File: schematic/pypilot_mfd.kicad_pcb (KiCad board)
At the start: 2 copper layers, 115.8 x 85.9 mm, 72 parts, among them J1 usb, J2 keypad, J3 Conn_01x02, J4 Conn_01x02, J5 jlx256160, J6 usb, J7 uart, Q1 Q_PMOS_GSD, Q2 Q_PMOS_GSD, Q3 Q_PMOS_DSG, SW1 BOOT/AP, U1 CH340G, U2 AMS1117-3.3, U3 ESP32-WROOM-32D, U5 ADM2587E, U6 LIS2DE12, U7 74AHC04, U8 BUZZER-freetronics_schematic, Y1 12mhz

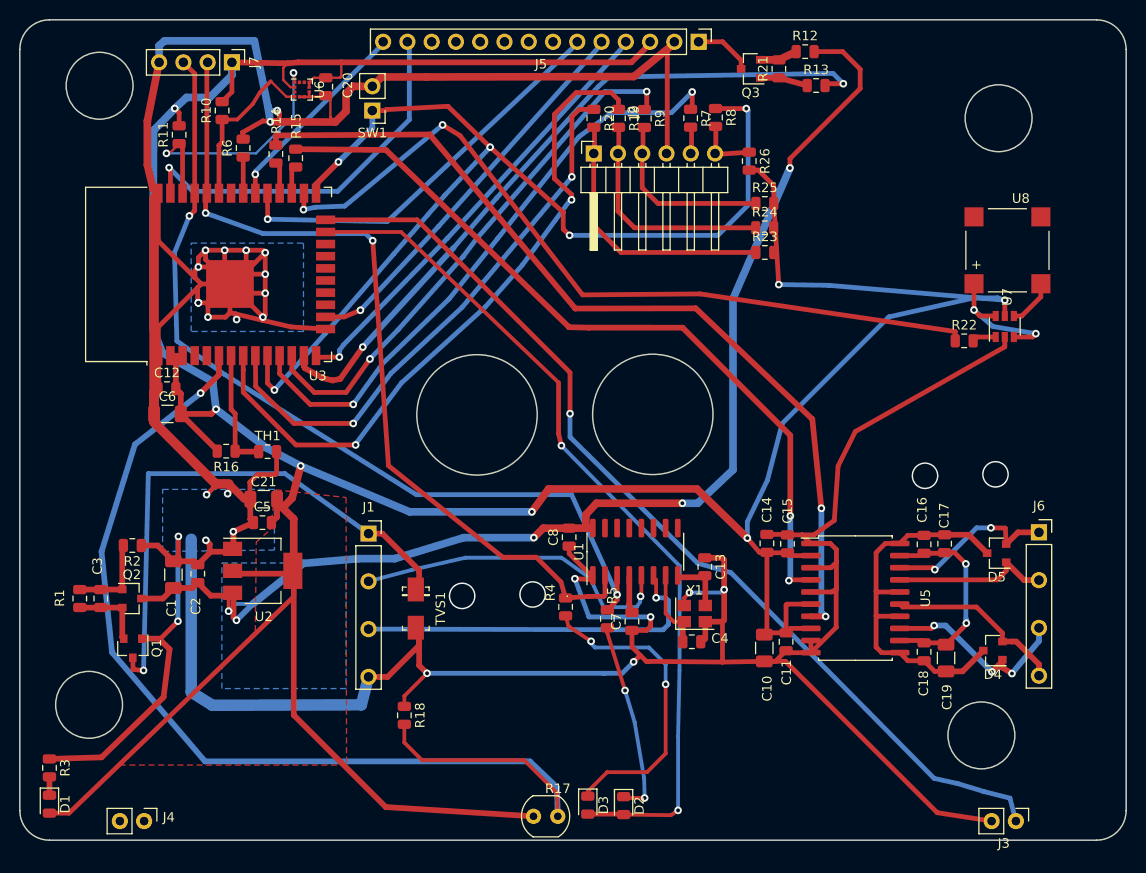
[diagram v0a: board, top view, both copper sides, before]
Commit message: many updates!
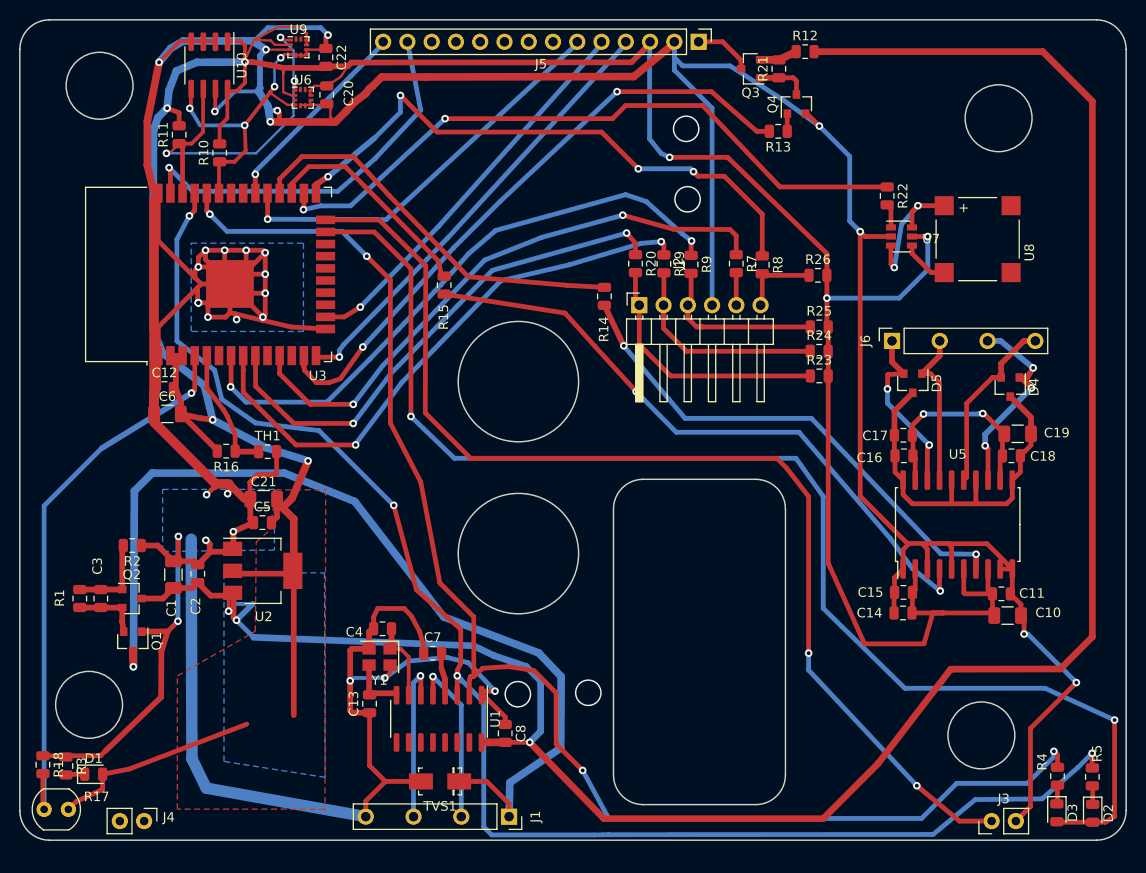
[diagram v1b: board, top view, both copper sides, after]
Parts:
- removed J7: uart, Connector_PinHeader_2.54mm:PinHeader_1x04_P2.54mm_Vertical
- removed R6: 1.2k, Resistor_SMD:R_0805_2012Metric
- removed SW1: BOOT/AP, Connector_PinHeader_2.54mm:PinHeader_1x02_P2.54mm_Vertical
- added C22: .1uF, Capacitor_SMD:C_0805_2012Metric, F.Cu at (44.9, 18.1)
- added Q4: Q_NMOS_GSD, pypilot_footprints:SOT-23_180, F.Cu at (94.1, 22.9)
- added U10: 24LC512, pypilot_footprints:SOIC-8_3.9x4.9mm_P1.27mm, F.Cu at (32.6, 18.9)
- added U9: LIS2DE12, pypilot_mfd_footprints:LGA-12_2x2mm_P0.5mm, F.Cu at (42.0, 17.0)
- U6: footprint pypilot_footprints:LGA-12_2x2mm_P0.5mm_90 -> pypilot_mfd_footprints:LGA-12_2x2mm_P0.5mm
- moved R4 54.5 mm to (121.4, 93.3)
- moved R5 53.4 mm to (125.1, 93.4)
- moved R17 51.2 mm to (16.6, 96.8), turned to 180 degrees
- moved D2 49.1 mm to (125.1, 97.2)
- moved D3 49.1 mm to (121.4, 97.1)
- moved R18 38.2 mm to (15.2, 92.1)
- moved C13 37.9 mm to (49.4, 85.7), turned to 90 degrees
- moved R14 37.5 mm to (74.0, 43.1), turned to 270 degrees
- moved Y1 33.3 mm to (50.5, 80.8), turned to 180 degrees
- moved J1 33.1 mm to (64.0, 97.5), turned to 270 degrees
- moved C4 32.4 mm to (50.8, 77.9), turned to 0 degrees
- moved D4 27.6 mm to (116.5, 52.6), turned to 90 degrees
- moved U1 26.7 mm to (56.7, 87.1), turned to 180 degrees
- moved C10 25.7 mm to (116.2, 76.5), turned to 180 degrees
- moved J6 25.3 mm to (104.1, 47.7), turned to 90 degrees
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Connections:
- R13 pad 1: Net-(Q3-Pad1) -> Net-(Q4-Pad1)
- U3 pad 10: PWR -> Net-(U3-Pad10)
- U3 pad 12: UP -> CS_SD
- U3 pad 31: Net-(R6-Pad1) -> MISO
- U3 pad 4: Net-(U3-Pad4) -> Net-(R17-Pad2)
- U3 pad 5: Net-(U3-Pad5) -> Net-(R16-Pad1)
- U3 pad 6: Net-(R17-Pad2) -> Net-(U3-Pad6)
- U3 pad 7: Net-(R16-Pad1) -> UP
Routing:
- net +5V: track 129.5 -> 225.0 mm, vias 5 -> 3
- net TX: track 91.6 -> 154.3 mm, vias 2 -> 4
- net RX: track 87.9 -> 146.7 mm, vias 2 -> 4
- net Net-(R17-Pad2): track 114.3 -> 59.2 mm
- net GND: track 554.9 -> 604.5 mm, vias 26 -> 31
- net +3V3: track 393.4 -> 345.3 mm
- net PWR: track 109.5 -> 62.3 mm, vias 5 -> 4
- net LEDS: track 90.2 -> 135.6 mm
- net Net-(J1-Pad1): track 56.9 -> 99.6 mm
- net Net-(R14-Pad2): track 92.7 -> 52.7 mm
- net TX1: track 3.33 -> 41.9 mm
- net Net-(D3-Pad1): track 32.9 -> 1.98 mm, vias 2 -> 0
- net Net-(J1-Pad3): track 37.8 -> 17.1 mm
- net RX1: track 3.19 -> 23.0 mm
- net Net-(D2-Pad1): track 20.6 -> 1.94 mm, vias 2 -> 0
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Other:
- outline, holes or cut-outs redrawn
- board text added: "pypilot mfd 0.4"
- board text removed: "pypilot mfd 0.3"

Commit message: update layout
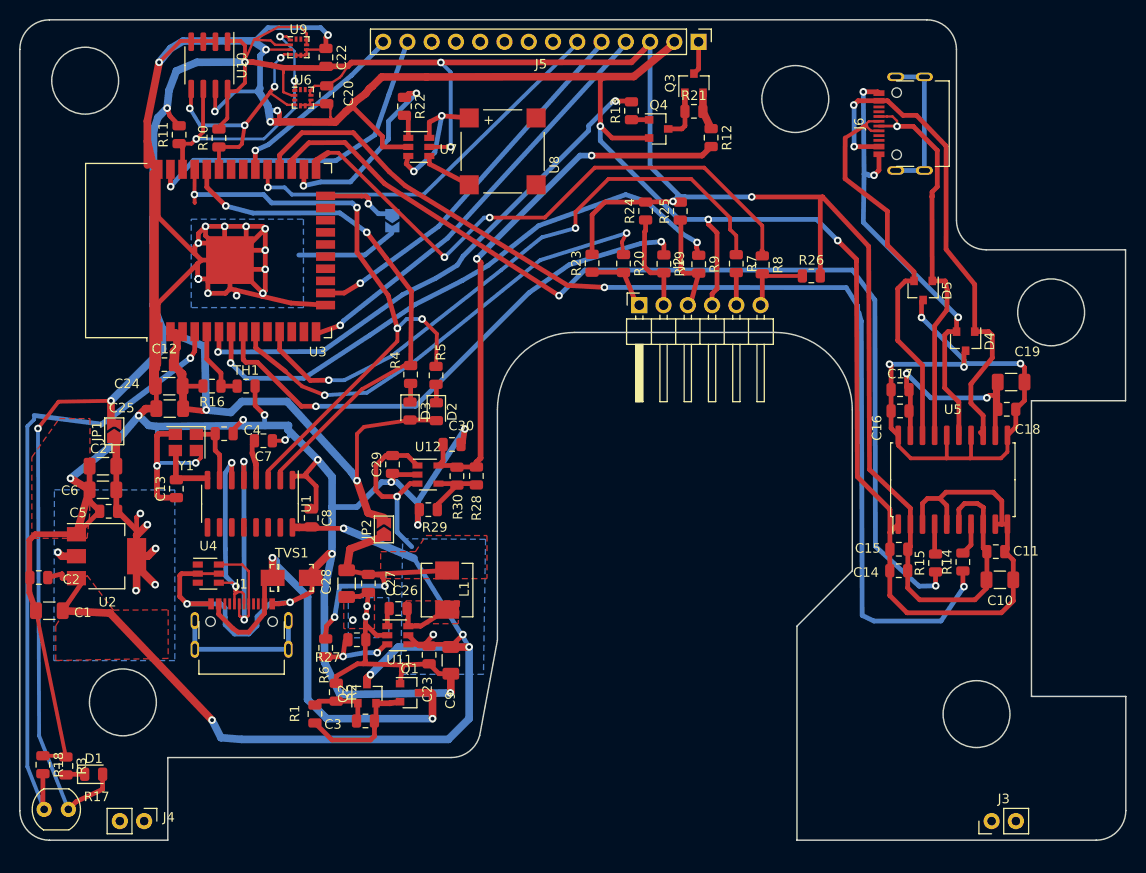
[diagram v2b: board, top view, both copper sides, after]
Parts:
- added C23: 100n, Capacitor_SMD:C_0805_2012Metric, F.Cu at (55.6, 80.6)
- added C24: 10uF, Capacitor_SMD:C_1206_3216Metric, F.Cu at (28.4, 52.5)
- added C25: 10uF, Capacitor_SMD:C_1206_3216Metric, F.Cu at (28.5, 54.8)
- added C26: 100n, Capacitor_SMD:C_0805_2012Metric, F.Cu at (52.4, 75.8)
- added C27: 100n, Capacitor_SMD:C_0805_2012Metric, F.Cu at (49.3, 73.1)
- added C28: 10uF, Capacitor_SMD:C_1206_3216Metric, F.Cu at (47.0, 73.1)
- added C29: 1uF, Capacitor_SMD:C_0805_2012Metric, F.Cu at (51.8, 60.7)
- added C30: 1uF, Capacitor_SMD:C_0805_2012Metric, F.Cu at (58.0, 58.6)
- added C9: 10uF, Capacitor_SMD:C_1206_3216Metric, F.Cu at (57.9, 81.2)
- added JP1: Jumper, Jumper:SolderJumper-2_P1.3mm_Open_TrianglePad1.0x1.5mm, F.Cu at (22.7, 57.2)
- added JP2: Jumper, Jumper:SolderJumper-2_P1.3mm_Open_TrianglePad1.0x1.5mm, F.Cu at (50.9, 67.5)
- added JP3: Jumper, Jumper:SolderJumper-2_P1.3mm_Open_TrianglePad1.0x1.5mm, B.Cu at (51.8, 35.1)
- added L1: 4.7uH, Inductor_SMD:L_Sunlord_MWSA0518_5.4x5.2mm, F.Cu at (57.5, 73.8)
- added R27: 22k, Resistor_SMD:R_0805_2012Metric, F.Cu at (48.1, 79.0)
- added R28: 100k, Resistor_SMD:R_0805_2012Metric, F.Cu at (60.6, 61.9)
- added R29: 22k, Resistor_SMD:R_0805_2012Metric, F.Cu at (55.6, 65.4)
- added R30: 100k, Resistor_SMD:R_0805_2012Metric, F.Cu at (58.6, 61.9)
- added R6: 51k, Resistor_SMD:R_0805_2012Metric, F.Cu at (44.8, 79.9)
- added U11: LMR50410, Package_TO_SOT_SMD:SOT-23-6, F.Cu at (52.4, 78.5)
- added U12: AP2127K-ADJ, Package_TO_SOT_SMD:SOT-23-5, F.Cu at (55.5, 61.7)
- added U4: SN65220, Package_TO_SOT_SMD:SOT-23-6, F.Cu at (32.5, 72.1)
- J1, J6: footprint pypilot_mfd_footprints:PinSocket_1x04_P2.54mm_Vertical -> pypilot_footprints:USB_C_Receptacle_Palconn_UTC16-G
- R12: value 47 -> 22
- R3: value 1.2k -> 1.5k
- moved D2 80.5 mm to (56.4, 55.1)
- moved R5 80.5 mm to (56.4, 51.3)
- moved D3 79.7 mm to (53.6, 55.1)
- moved R4 79.7 mm to (53.7, 51.2)
- moved R15 59.1 mm to (108.7, 71.0), turned to 90 degrees
- moved R22 51.4 mm to (53.1, 23.2)
- moved U7 51.4 mm to (54.6, 27.4)
- moved U8 50.6 mm to (63.4, 27.9)
- moved R14 46.7 mm to (111.5, 70.9), turned to 90 degrees
- moved J1 34.3 mm to (36.0, 77.8), turned to 0 degrees
- moved C3 30.5 mm to (49.0, 87.5), turned to 0 degrees
- moved C8 30.3 mm to (43.3, 66.3)
- moved C13 30.3 mm to (29.2, 63.2)
- moved Y1 30.3 mm to (30.2, 58.4)
- moved U1 30.0 mm to (36.9, 64.6)
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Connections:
- net Net-(J5-Pad1) renamed BACKLIGHT
- C21 pad 2: +3V3 -> Net-(C21-Pad2)
- C5 pad 2: +3V3 -> Net-(C21-Pad2)
- C6 pad 2: +3V3 -> Net-(C21-Pad2)
- D2 pad 2: LEDS -> +3V3
- D3 pad 2: LEDS -> +3V3
- J3 pad 2: GND -> Net-(J3-Pad2)
- Q1 pad 3: Net-(J1-Pad1) -> Net-(J1-PadA4)
- R12 pad 2: +5V -> Net-(C30-Pad2)
- TVS1 pad 1: Net-(J1-Pad1) -> Net-(J1-PadA4)
- U1 pad 5: Net-(J1-Pad2) -> Net-(J1-PadA6)
- U1 pad 6: Net-(J1-Pad3) -> Net-(J1-PadA7)
- U2 pad 2: +3V3 -> Net-(C21-Pad2)
- U3 pad 13: LEDA -> Net-(U3-Pad13)
- U3 pad 23: LEDS -> Net-(U3-Pad23)
- U3 pad 24: Net-(J3-Pad1) -> Net-(JP3-Pad1)
- U3 pad 6: Net-(U3-Pad6) -> LEDA
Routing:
- net LEDS: track 135.6 -> 0.00 mm, vias 2 -> 0
- net Net-(J3-Pad1): track 115.7 -> 0.00 mm, vias 2 -> 0
- net Net-(J1-Pad1): track 99.6 -> 0.00 mm, vias 1 -> 0
- net RX: track 146.7 -> 54.5 mm, vias 4 -> 2
- net +5V: track 225.0 -> 134.3 mm, vias 3 -> 7
- net TX: track 154.3 -> 65.0 mm
- net RX1: track 23.0 -> 105.9 mm, vias 0 -> 2
- net TX1: track 41.9 -> 116.3 mm, vias 0 -> 2
- net Net-(R15-Pad2): track 67.6 -> 3.16 mm, vias 2 -> 0
- net Net-(C30-Pad2): track 0.00 -> 58.0 mm, vias 0 -> 2
- net GND: track 604.5 -> 660.8 mm, vias 31 -> 39
- net +3V3: track 345.3 -> 396.0 mm, vias 7 -> 10
- net BUZZER: track 70.7 -> 20.1 mm
- net Net-(R14-Pad2): track 52.7 -> 3.38 mm, vias 2 -> 0
- net Net-(J1-PadA4): track 0.00 -> 48.8 mm, vias 0 -> 2
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- added copper zone on F.Cu, net +5V
- added copper zone on F.Cu, net GND
- added copper zone on B.Cu, net Net-(C21-Pad2)
- added copper zone on F.Cu, net Net-(C26-Pad1)
- added copper zone on F.Cu, net Net-(C27-Pad2)
- removed copper zone on F.Cu, net +3V3
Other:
- outline, holes or cut-outs redrawn
- board text added: "pypilot mfd 0.42"
- board text removed: "pypilot mfd 0.4"
